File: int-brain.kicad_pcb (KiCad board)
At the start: 2 copper layers, 107 x 79.5 mm, 123 parts, among them J1 Top, J10 2MB, J11 1MB, J12 1MA, J13 1MA_ENC, J14 1MB_ENC, J15 2MA_ENC, J16 MPU9250, J17 VBATT_SELECT, J18 I2C0, J2 Bottom, J3 PWR, J4 PWR, J5 USB_A, J6 2MB_ENC, J7 I2C1, J8 UART0, J9 2MA, SW1 ON/OFF, U1 PCA9635, U10 TPS5450DDA, U11 DRV8251ADDAR, U12 INA139, U13 AMS1117-3.3, U2 ESP32-DevKitC, U3 DRV8251ADDAR, U4 INA139, U5 DRV8251ADDAR, U6 INA139, U7 TPS5450DDA, U8 DRV8251ADDAR, U9 INA139

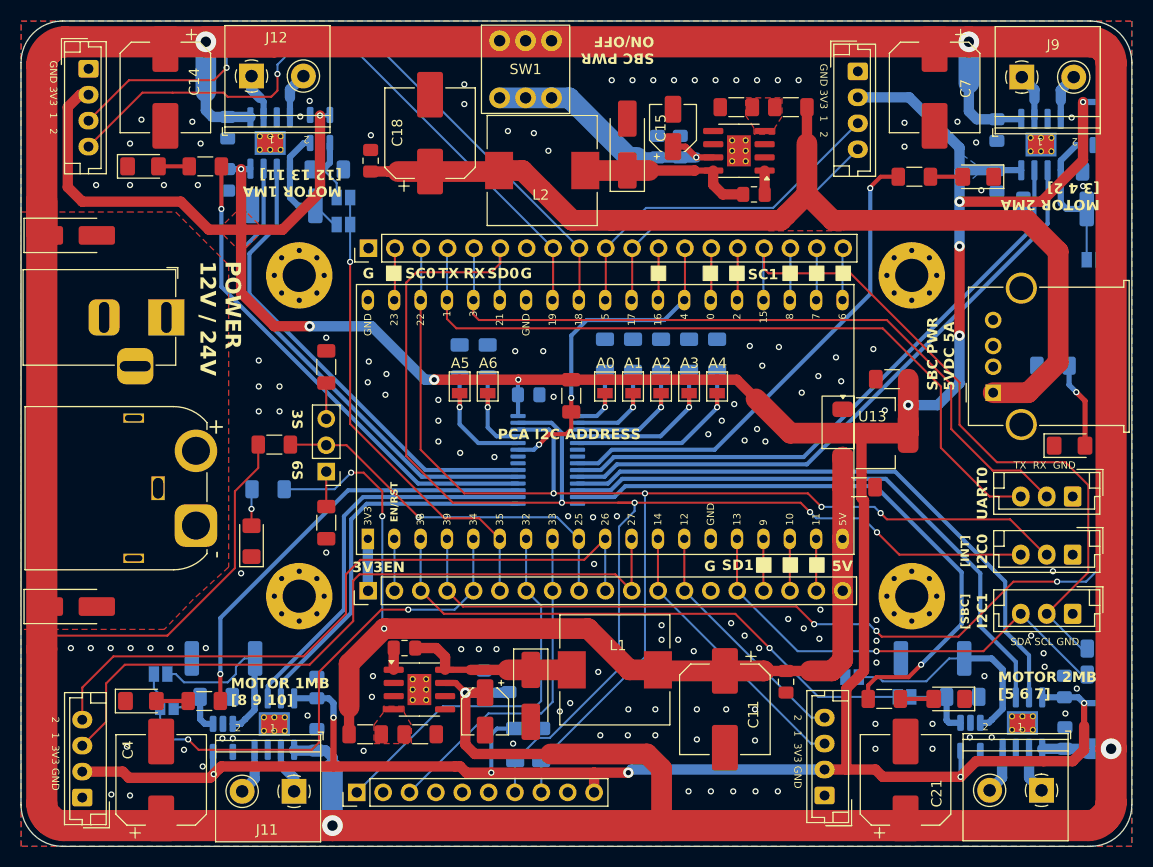
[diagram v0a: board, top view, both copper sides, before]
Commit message: finally done?
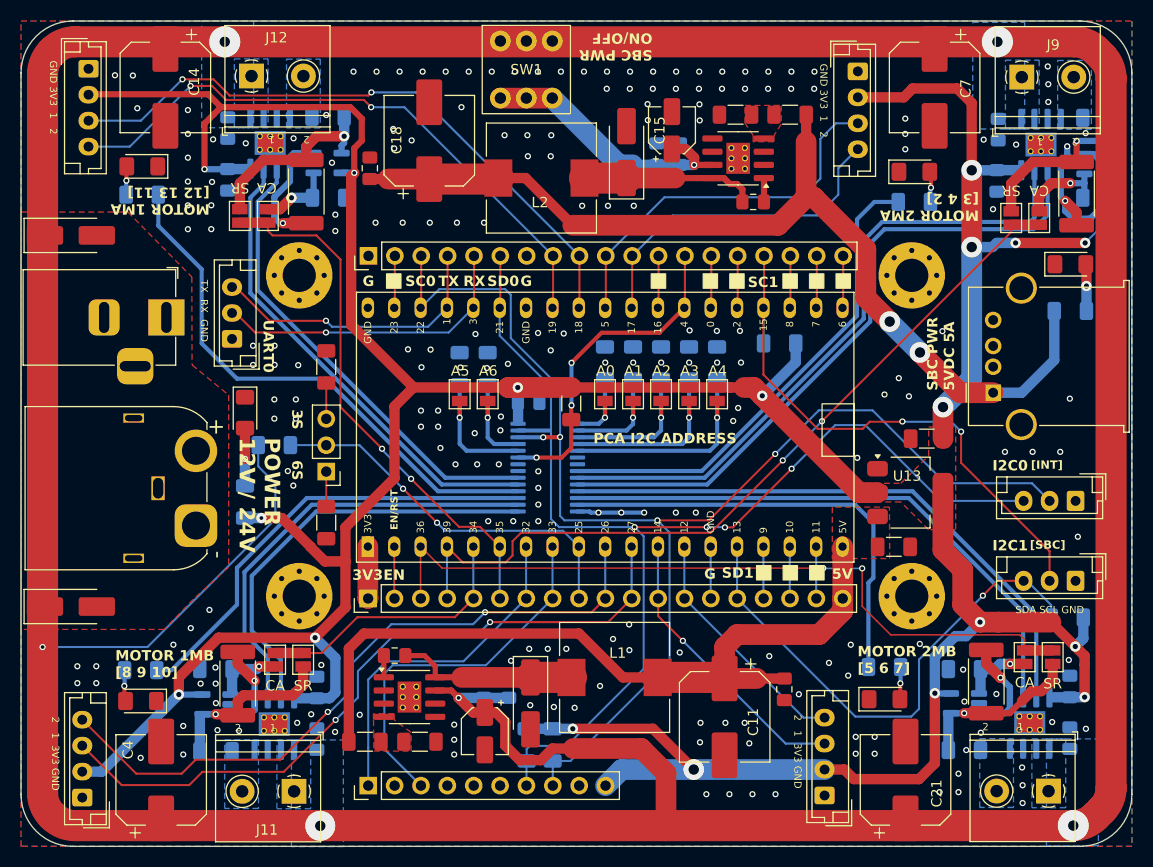
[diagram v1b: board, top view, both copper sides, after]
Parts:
- added R34: R_TRIP, Resistor_SMD:R_1206_3216Metric_Pad1.30x1.75mm_HandSolder, B.Cu at (124.9, 70.9)
- added R35: R_TRIP, Resistor_SMD:R_1206_3216Metric_Pad1.30x1.75mm_HandSolder, B.Cu at (114.1, 132.0)
- added R36: R_TRIP, Resistor_SMD:R_1206_3216Metric_Pad1.30x1.75mm_HandSolder, B.Cu at (199.2, 71.0)
- added R37: R_TRIP, Resistor_SMD:R_1206_3216Metric_Pad1.30x1.75mm_HandSolder, B.Cu at (186.2, 131.9)
- JP10, JP11, JP8, JP9: value PA -> CA; moved to F.Cu
- JP12, JP13, JP14, JP15: moved to F.Cu
- R1, R2, R3, R5, R8: moved to B.Cu
- R14: value 470R -> 220R
- R17, R19, R23, R27: value 10mR -> R_SHUNT; moved to F.Cu
- R18, R20, R24, R28: value 24k -> R_GAIN
- moved J8 82.4 mm to (115.7, 92.3), turned to 90 degrees
- moved R32 42.9 mm to (168.4, 92.7)
- moved JP15 19.4 mm to (194.7, 123.0), turned to 90 degrees
- moved D6 17.5 mm to (196.4, 85.1)
- moved JP13 13.8 mm to (122.5, 123.2), turned to 90 degrees
- moved D7 12.4 mm to (116.9, 99.4), turned to -90 degrees
- moved JP11 12.2 mm to (192.0, 123.0), turned to -90 degrees
- moved JP9 11.4 mm to (119.8, 123.2), turned to -90 degrees
- moved JP12 10.0 mm to (116.4, 80.5), turned to -90 degrees
- moved JP14 8.89 mm to (190.7, 80.7), turned to -90 degrees
- moved JP8 7.49 mm to (119.1, 80.5), turned to 90 degrees
- moved JP10 7.32 mm to (193.4, 80.7), turned to 90 degrees
- moved R2 6.81 mm to (106.8, 124.2)
- moved C26 6.67 mm to (179.4, 112.3)
- moved R1 6.66 mm to (107.0, 78.4)
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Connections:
- JP10 pad 1: Net-(JP10-A) -> 2MA_SENSE
- JP10 pad 2: 2MA_SENSE -> /motor-driver-3/I_SEN_CA
- JP11 pad 1: Net-(JP11-A) -> 2MB_SENSE
- JP11 pad 2: 2MB_SENSE -> /motor-driver-4/I_SEN_CA
- JP12 pad 1: /motor-driver-1/IPROPI -> /motor-driver-1/I_SEN_SR
- JP13 pad 1: /motor-driver-2/IPROPI -> /motor-driver-2/I_SEN_SR
- JP14 pad 1: /motor-driver-3/IPROPI -> /motor-driver-3/I_SEN_SR
- JP15 pad 1: /motor-driver-4/IPROPI -> /motor-driver-4/I_SEN_SR
- JP8 pad 1: Net-(JP8-A) -> 1MA_SENSE
- JP8 pad 2: 1MA_SENSE -> /motor-driver-1/I_SEN_CA
- JP9 pad 1: Net-(JP9-A) -> 1MB_SENSE
- JP9 pad 2: 1MB_SENSE -> /motor-driver-2/I_SEN_CA
- R14 pad 1: VSS -> +3.3V
- R17 pad 2: GND -> /motor-driver-2/I_SEN_SR
- R18 pad 1: Net-(JP9-A) -> /motor-driver-2/I_SEN_CA
- R19 pad 2: GND -> /motor-driver-3/I_SEN_SR
- R20 pad 1: Net-(JP10-A) -> /motor-driver-3/I_SEN_CA
- R23 pad 2: GND -> /motor-driver-1/I_SEN_SR
- R24 pad 1: Net-(JP8-A) -> /motor-driver-1/I_SEN_CA
- R27 pad 2: GND -> /motor-driver-4/I_SEN_SR
- R28 pad 1: Net-(JP11-A) -> /motor-driver-4/I_SEN_CA
- U12 pad 1: Net-(JP11-A) -> /motor-driver-4/I_SEN_CA
- U12 pad 4: GND -> /motor-driver-4/I_SEN_SR
- U4 pad 1: Net-(JP9-A) -> /motor-driver-2/I_SEN_CA
- U4 pad 4: GND -> /motor-driver-2/I_SEN_SR
- U6 pad 1: Net-(JP10-A) -> /motor-driver-3/I_SEN_CA
- U6 pad 4: GND -> /motor-driver-3/I_SEN_SR
- U9 pad 1: Net-(JP8-A) -> /motor-driver-1/I_SEN_CA
- U9 pad 4: GND -> /motor-driver-1/I_SEN_SR
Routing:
- net VS: track 477.1 -> 423.8 mm, vias 5 -> 6
- net /TX0: track 72.7 -> 27.7 mm, vias 0 -> 1
- net /RX0: track 71.4 -> 29.7 mm, vias 0 -> 1
- net 2MA_SENSE: track 108.6 -> 77.4 mm, vias 3 -> 2
- net SDA0: track 142.4 -> 115.5 mm
- net VSS: track 101.6 -> 75.3 mm, vias 3 -> 0
- net 1MB_SENSE: track 51.8 -> 26.3 mm, vias 2 -> 0
- net /motor-driver-3/I_SEN_SR: track 0.00 -> 18.8 mm, vias 0 -> 1
- net /motor-driver-1/I_SEN_SR: track 0.00 -> 18.8 mm, vias 0 -> 1
- net /motor-driver-2/I_SEN_SR: track 0.00 -> 16.7 mm, vias 0 -> 1
- net /motor-driver-4/I_SEN_SR: track 0.00 -> 15.9 mm, vias 0 -> 1
- net 2MB_SENSE: track 57.1 -> 72.8 mm, vias 1 -> 2
- net /2MB_EN: track 58.6 -> 43.3 mm, vias 1 -> 0
- net GND: track 0.00 -> 14.3 mm, vias 139 -> 215
- net /SCL1: track 68.6 -> 55.2 mm, vias 0 -> 2
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- added copper zone on B.Cu, net /1MA1
- added copper zone on B.Cu, net /1MA2
- added copper zone on B.Cu, net /1MB1
- added copper zone on B.Cu, net /1MB2
- added copper zone on B.Cu, net /2MA1
- added copper zone on B.Cu, net /2MA2
- added copper zone on B.Cu, net /2MB1
- added copper zone on B.Cu, net /2MB2
- added copper zone on B.Cu, net VS
- added copper zone on F.Cu, net VSS
- removed copper zone on B.Cu, net +3.3V
- removed copper zone on F.Cu, net /buck2/VOUT
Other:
- outline, holes or cut-outs redrawn
- board text added: "107 mm x 79.5 mm"
